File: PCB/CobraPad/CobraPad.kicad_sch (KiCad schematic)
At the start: 35 parts, among them SW1 SW_Push, SW2 SW_Push, SW3 SW_Push, SW4 SW_Push, SW5 SW_Push, SW6 SW_Push, SW7 SW_Push, SW8 SW_Push, SW9 RotaryEncoder_Switch, U1 MOUDLE-SEEEDUINO-XIAO, U2 ER_OLEDM0.91_1x-I2C

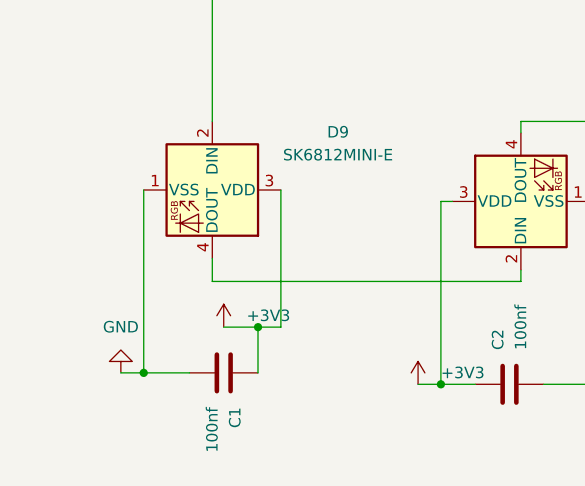
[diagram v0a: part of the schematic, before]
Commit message: Scamatic Done
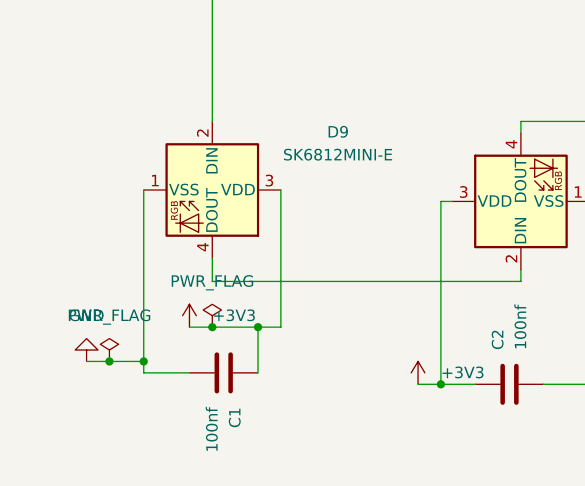
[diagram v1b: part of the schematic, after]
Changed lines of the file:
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@@
 	(paper "A4")
 	(junction
+		(at 24.13 149.86)
+		(diameter 0)
+		(color 0 0 0 0)
+	)
+	(junction
 		(at 106.68 151.13)
 		(diameter 0)
@@
 	)
 	(junction
-		(at 27.94 151.13)
-		(diameter 0)
-		(color 0 0 0 0)
-	)
-	(junction
 		(at 118.11 152.4)
 		(diameter 0)
@@
 	)
 	(junction
-		(at 246.38 149.86)
+		(at 40.64 146.05)
 		(diameter 0)
 		(color 0 0 0 0)
 	)
 	(junction
-		(at 40.64 146.05)
+		(at 27.94 149.86)
+		(diameter 0)
+		(color 0 0 0 0)
+	)
+	(junction
+		(at 246.38 149.86)
 		(diameter 0)
 		(color 0 0 0 0)
@@
 	)
 	(junction
+		(at 35.56 146.05)
+		(diameter 0)
+		(color 0 0 0 0)
+	)
+	(junction
 		(at 91.44 151.13)
 		(diameter 0)
@@
 	(wire
 		(pts
+			(xy 35.56 146.05) (xy 40.64 146.05)
+		)
+		(stroke
+			(width 0)
+			(type default)
+		)
+	)
+	(wire
+		(pts
+			(xy 27.94 149.86) (xy 27.94 151.13)
+		)
+		(stroke
+			(width 0)
+			(type default)
+		)
+	)
+	(wire
+		(pts
 			(xy 45.72 40.64) (xy 50.8 40.64)
 		)
@@
 	(wire
 		(pts
-			(xy 36.83 146.05) (xy 40.64 146.05)
+			(xy 33.02 146.05) (xy 35.56 146.05)
 		)
 		(stroke
@@
 	(wire
 		(pts
-			(xy 27.94 130.81) (xy 27.94 151.13)
+			(xy 27.94 130.81) (xy 27.94 149.86)
 		)
 		(stroke
@@
 	(wire
 		(pts
+			(xy 24.13 149.86) (xy 27.94 149.86)
+		)
+		(stroke
+			(width 0)
+			(type default)
+		)
+	)
+	(wire
+		(pts
 			(xy 19.05 30.48) (xy 22.86 30.48)
 		)
@@
 	(wire
 		(pts
-			(xy 25.4 151.13) (xy 27.94 151.13)
+			(xy 21.59 149.86) (xy 24.13 149.86)
 		)
 		(stroke
@@
 	)
 	(symbol
+		(lib_id "power:PWR_FLAG")
+		(at 35.56 146.05 0)
+		(unit 1)
+		(body_style 1)
+		(exclude_from_sim no)
+		(in_bom yes)
+		(on_board yes)
+		(in_pos_files yes)
+		(dnp no)
+		(fields_autoplaced yes)
+		(property "Reference" "#FLG03"
+			(at 35.56 144.145 0)
+			(hide yes)
+			(show_name no)
+			(do_not_autoplace no)
+			(effects
+				(font
+					(size 1.27 1.27)
+				)
+			)
+		)
+		(property "Value" "PWR_FLAG"
+			(at 35.56 140.97 0)
+			(show_name no)
+			(do_not_autoplace no)
+			(effects
+				(font
+					(size 1.27 1.27)
+				)
+			)
+		)
+		(property "Footprint" ""
+			(at 35.56 146.05 0)
+			(hide yes)
+			(show_name no)
+			(do_not_autoplace no)
+			(effects
+				(font
+					(size 1.27 1.27)
+				)
+			)
+		)
+		(property "Datasheet" ""
+			(at 35.56 146.05 0)
+			(hide yes)
+			(show_name no)
+			(do_not_autoplace no)
+			(effects
+				(font
+					(size 1.27 1.27)
+				)
+			)
+		)
+		(property "Description" "Special symbol for telling ERC where power comes from"
+			(at 35.56 146.05 0)
+			(hide yes)
+			(show_name no)
+			(do_not_autoplace no)
+			(effects
+				(font
+					(size 1.27 1.27)
+				)
+			)
+		)
+		(pin "1"
+		)
+		(instances
+			(project "CobraPad"
+				(path "/2a034d3a-ddfe-40b9-a8fa-eac088730dee"
+					(reference "#FLG03")
+					(unit 1)
+				)
+			)
+		)
+	)
+	(symbol
 		(lib_id "power:+3V3")
 		(at 171.45 151.13 0)
@@
 	(symbol
 		(lib_id "power:GND")
-		(at 25.4 151.13 180)
+		(at 21.59 149.86 180)
 		(unit 1)
 		(body_style 1)
@@
 		(fields_autoplaced yes)
 		(property "Reference" "#PWR01"
-			(at 25.4 144.78 0)
+			(at 21.59 143.51 0)
 			(hide yes)
 			(show_name no)
@@
 		)
 		(property "Value" "GND"
-			(at 25.4 146.05 0)
+			(at 21.59 144.78 0)
 			(show_name no)
 			(do_not_autoplace no)
@@
 		)
 		(property "Footprint" ""
-			(at 25.4 151.13 0)
+			(at 21.59 149.86 0)
 			(hide yes)
 			(show_name no)
@@
 		)
 		(property "Datasheet" ""
-			(at 25.4 151.13 0)
+			(at 21.59 149.86 0)
 			(hide yes)
 			(show_name no)
@@
 		)
 		(property "Description" "Power symbol creates a global label with name \"GND\" , ground"
-			(at 25.4 151.13 0)
+			(at 21.59 149.86 0)
 			(hide yes)
 			(show_name no)
@@
 	(symbol
 		(lib_id "power:+3V3")
-		(at 36.83 146.05 0)
+		(at 33.02 146.05 0)
 		(unit 1)
 		(body_style 1)
@@
 		(fields_autoplaced yes)
 		(property "Reference" "#PWR017"
-			(at 36.83 149.86 0)
+			(at 33.02 149.86 0)
 			(hide yes)
 			(show_name no)
@@
 		)
 		(property "Value" "+3V3"
-			(at 39.37 144.7799 0)
+			(at 35.56 144.7799 0)
 			(show_name no)
 			(do_not_autoplace no)
@@
 		)
 		(property "Footprint" ""
-			(at 36.83 146.05 0)
+			(at 33.02 146.05 0)
 			(hide yes)
 			(show_name no)
@@
 		)
 		(property "Datasheet" ""
-			(at 36.83 146.05 0)
+			(at 33.02 146.05 0)
 			(hide yes)
 			(show_name no)
@@
 		)
 		(property "Description" "Power symbol creates a global label with name \"+3V3\""
-			(at 36.83 146.05 0)
+			(at 33.02 146.05 0)
 			(hide yes)
 			(show_name no)
@@
 					(unit 1)
 				)
+			)
+		)
+	)
+	(symbol
+		(lib_id "power:PWR_FLAG")
+		(at 24.13 149.86 0)
+		(unit 1)
+		(body_style 1)
+		(exclude_from_sim no)
+		(in_bom yes)
+		(on_board yes)
+		(in_pos_files yes)
+		(dnp no)
+		(fields_autoplaced yes)
+		(property "Reference" "#FLG04"
+			(at 24.13 147.955 0)
+			(hide yes)
+			(show_name no)
+			(do_not_autoplace no)
+			(effects
+				(font
+					(size 1.27 1.27)
+				)
+			)
+		)
+		(property "Value" "PWR_FLAG"
+			(at 24.13 144.78 0)
+			(show_name no)
+			(do_not_autoplace no)
+			(effects
+				(font
+					(size 1.27 1.27)
+				)
+			)
+		)
+		(property "Footprint" ""
+			(at 24.13 149.86 0)
+			(hide yes)
+			(show_name no)
+			(do_not_autoplace no)
+			(effects
+				(font
+					(size 1.27 1.27)
+				)
+			)
+		)
+		(property "Datasheet" ""
+			(at 24.13 149.86 0)
+			(hide yes)
+			(show_name no)
+			(do_not_autoplace no)
+			(effects
+				(font
+					(size 1.27 1.27)
+				)
+			)
+		)
+		(property "Description" "Special symbol for telling ERC where power comes from"
+			(at 24.13 149.86 0)
+			(hide yes)
+			(show_name no)
+			(do_not_autoplace no)
+			(effects
+				(font
+					(size 1.27 1.27)
+				)
+			)
+		)
+		(pin "1"
+		)
+		(instances
+			(project "CobraPad"
+				(path "/2a034d3a-ddfe-40b9-a8fa-eac088730dee"
+					(reference "#FLG04")
+					(unit 1)
+				)

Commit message: PCB done
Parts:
- C1, C2, C3, C4, C5, C6, C7, C8: footprint (none) -> Capacitor_SMD:C_0603_1608Metric
- SW1, SW2, SW3, SW4, SW5, SW6, SW7, SW8: footprint (none) -> Button_Switch_Keyboard:SW_Cherry_MX_1.00u_Plate
- SW9: footprint (none) -> Rotary_Encoder:RotaryEncoder_Alps_EC11E-Switch_Vertical_H20mm
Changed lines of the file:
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@@
 			)
 		)
-		(property "Footprint" ""
+		(property "Footprint" "Button_Switch_Keyboard:SW_Cherry_MX_1.00u_Plate"
 			(at 27.94 25.4 0)
 			(hide yes)
@@
 			)
 		)
-		(property "Footprint" ""
+		(property "Footprint" "Capacitor_SMD:C_0603_1608Metric"
 			(at 93.98 152.0952 0)
 			(hide yes)
@@
 			)
 		)
-		(property "Footprint" ""
+		(property "Footprint" "Button_Switch_Keyboard:SW_Cherry_MX_1.00u_Plate"
 			(at 27.94 15.24 0)
 			(hide yes)
@@
 			)
 		)
-		(property "Footprint" ""
+		(property "Footprint" "Button_Switch_Keyboard:SW_Cherry_MX_1.00u_Plate"
 			(at 27.94 35.56 0)
 			(hide yes)
@@
 			)
 		)
-		(property "Footprint" ""
+		(property "Footprint" "Capacitor_SMD:C_0603_1608Metric"
 			(at 185.42 150.1648 0)
 			(hide yes)
@@
 			)
 		)
-		(property "Footprint" ""
+		(property "Footprint" "Capacitor_SMD:C_0603_1608Metric"
 			(at 33.02 152.0952 0)
 			(hide yes)
@@
 			)
 		)
-		(property "Footprint" ""
+		(property "Footprint" "Capacitor_SMD:C_0603_1608Metric"
 			(at 207.01 152.0952 0)
 			(hide yes)
@@
 			)
 		)
-		(property "Footprint" ""
+		(property "Footprint" "Button_Switch_Keyboard:SW_Cherry_MX_1.00u_Plate"
 			(at 74.93 54.61 0)
 			(hide yes)
@@
 			)
 		)
-		(property "Footprint" ""
+		(property "Footprint" "Capacitor_SMD:C_0603_1608Metric"
 			(at 72.39 151.4348 0)
 			(hide yes)
@@
 			)
 		)
-		(property "Footprint" ""
+		(property "Footprint" "Capacitor_SMD:C_0603_1608Metric"
 			(at 243.84 148.8948 0)
 			(hide yes)
@@
 			)
 		)
-		(property "Footprint" ""
+		(property "Footprint" "Button_Switch_Keyboard:SW_Cherry_MX_1.00u_Plate"
 			(at 27.94 46.99 0)
 			(hide yes)
@@
 			)
 		)
-		(property "Footprint" ""
+		(property "Footprint" "Capacitor_SMD:C_0603_1608Metric"
 			(at 129.54 151.4348 0)
 			(hide yes)
@@
 			)
 		)
-		(property "Footprint" ""
+		(property "Footprint" "Rotary_Encoder:RotaryEncoder_Alps_EC11E-Switch_Vertical_H20mm"
 			(at 218.186 86.36 0)
 			(hide yes)
@@
 			)
 		)
-		(property "Footprint" ""
+		(property "Footprint" "Button_Switch_Keyboard:SW_Cherry_MX_1.00u_Plate"
 			(at 74.93 16.51 0)
 			(hide yes)
@@
 			)
 		)
-		(property "Footprint" ""
+		(property "Footprint" "Capacitor_SMD:C_0603_1608Metric"
 			(at 152.4 152.0952 0)
 			(hide yes)
@@
 			)
 		)
-		(property "Footprint" ""
+		(property "Footprint" "Button_Switch_Keyboard:SW_Cherry_MX_1.00u_Plate"
 			(at 74.93 41.91 0)
 			(hide yes)
@@
 			)
 		)
-		(property "Footprint" ""
+		(property "Footprint" "Button_Switch_Keyboard:SW_Cherry_MX_1.00u_Plate"
 			(at 74.93 29.21 0)
 			(hide yes)
